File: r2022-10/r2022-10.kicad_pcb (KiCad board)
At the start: 4 copper layers, 100 x 80 mm, 137 parts, among them J1 Conn_01x03_Male, J2 USB_A male UP, J3 USB_B_Micro (up), J4 USB_A (female down), J5 USB_A_Stacked, J6 USB_A_Stacked, J7 USB_A_Stacked, J8 Conn_01x06, Q1 HSM6115, Q2 S8550, Q3 AO3401A, Q4 S8550, U1 2k i2c eeprom, U10 APL3511C, U11 NUP4202, U12 NUP4202, U13 NUP4202, U14 NUP4202, U15 NUP4202, U16 NUP4202, U17 NUP4202, U18 SiC437AED, U19 AMS1117-33, U2 NUP4202, U3 USB2517, U4 APL3511C, U5 APL3511C, U6 APL3511C, U7 APL3511C, U8 APL3511C, U9 APL3511C, Y1 24MHz

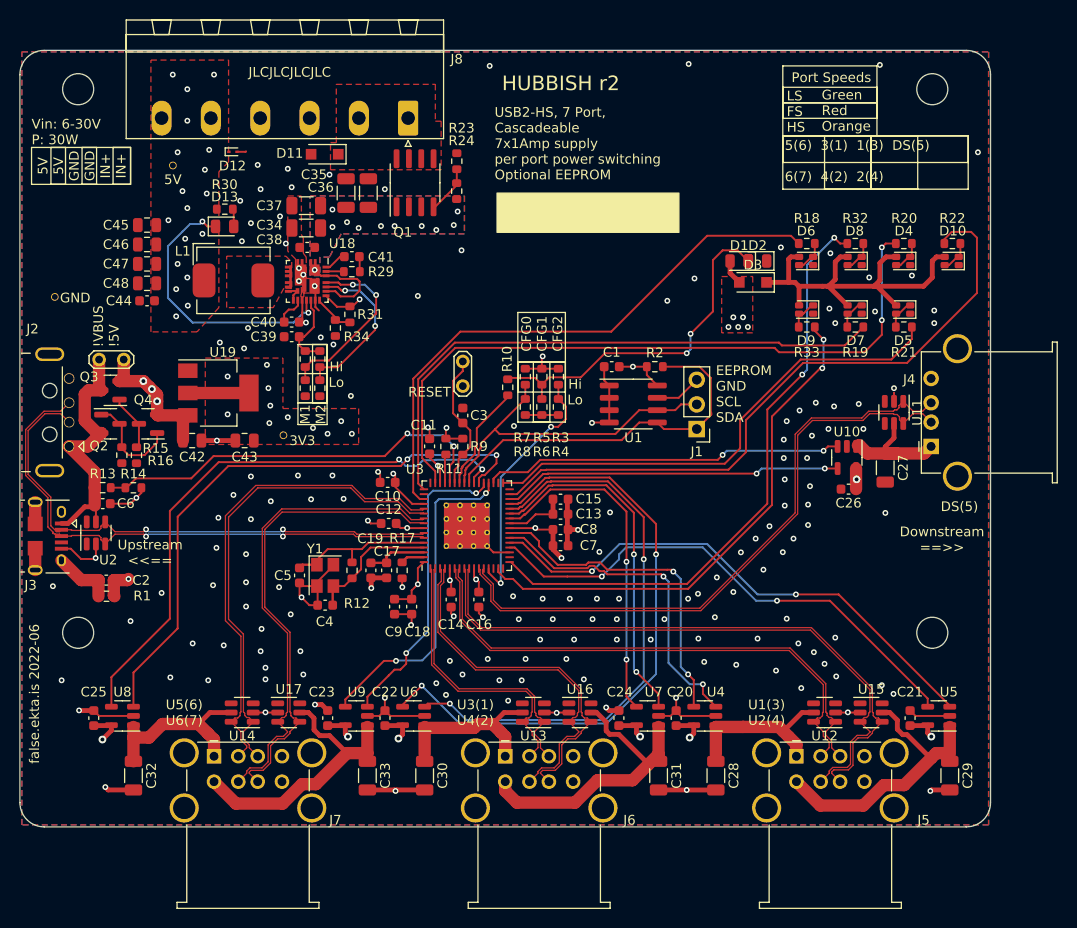
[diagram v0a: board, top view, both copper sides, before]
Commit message: r3: save all laast edits too
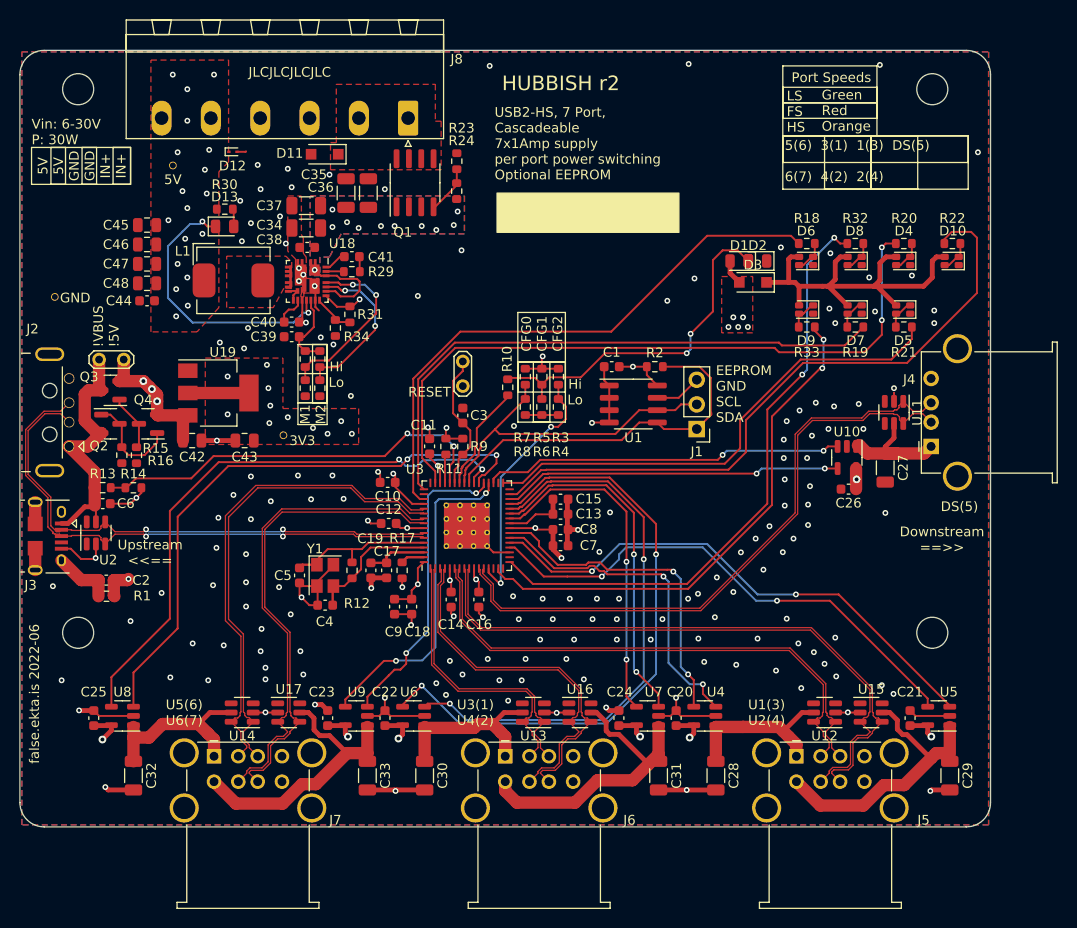
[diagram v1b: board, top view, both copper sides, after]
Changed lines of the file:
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@@
       (disableapertmacros false)
       (usegerberextensions false)
-      (usegerberattributes true)
+      (usegerberattributes false)
       (usegerberadvancedattributes true)
       (creategerberjobfile true)
@@
     (fp_line (start -1.6 -0.8) (end 1.6 -0.8) (layer "F.Fab") (width 0.1))
     (fp_line (start -1.6 0.8) (end -1.6 -0.8) (layer "F.Fab") (width 0.1))
-    (pad "1" smd roundrect (at -1.475 0 90) (size 1.15 1.8) (layers "F.Cu" "F.Paste" "F.Mask") (roundrect_rratio 0.217391)
+    (pad "1" smd roundrect (at -1.475 0 90) (size 1.15 1.8) (layers "F.Cu" "F.Paste" "F.Mask") (roundrect_rratio 0.2173913043)
       (net 14 "+VDC") (pintype "passive"))
-    (pad "2" smd roundrect (at 1.475 0 90) (size 1.15 1.8) (layers "F.Cu" "F.Paste" "F.Mask") (roundrect_rratio 0.217391)
+    (pad "2" smd roundrect (at 1.475 0 90) (size 1.15 1.8) (layers "F.Cu" "F.Paste" "F.Mask") (roundrect_rratio 0.2173913043)
       (net 1 "GND") (pintype "passive"))
     (model "${KICAD6_3DMODEL_DIR}/Capacitor_SMD.3dshapes/C_1206_3216Metric.wrl"
@@
     (fp_line (start 1.6 0.8) (end -1.6 0.8) (layer "F.Fab") (width 0.1))
     (fp_line (start -1.6 -0.8) (end 1.6 -0.8) (layer "F.Fab") (width 0.1))
-    (pad "1" smd roundrect (at -1.475 0 270) (size 1.15 1.8) (layers "F.Cu" "F.Paste" "F.Mask") (roundrect_rratio 0.217391)
+    (pad "1" smd roundrect (at -1.475 0 270) (size 1.15 1.8) (layers "F.Cu" "F.Paste" "F.Mask") (roundrect_rratio 0.2173913043)
       (net 9 "/downstream-port-power/VBUS2") (pintype "passive"))
-    (pad "2" smd roundrect (at 1.475 0 270) (size 1.15 1.8) (layers "F.Cu" "F.Paste" "F.Mask") (roundrect_rratio 0.217391)
+    (pad "2" smd roundrect (at 1.475 0 270) (size 1.15 1.8) (layers "F.Cu" "F.Paste" "F.Mask") (roundrect_rratio 0.2173913043)
       (net 1 "GND") (pintype "passive"))
     (model "${KICAD6_3DMODEL_DIR}/Capacitor_SMD.3dshapes/C_1206_3216Metric.wrl"
@@
     (fp_line (start 1.6 -0.8) (end 1.6 0.8) (layer "F.Fab") (width 0.1))
     (fp_line (start -1.6 0.8) (end -1.6 -0.8) (layer "F.Fab") (width 0.1))
-    (pad "1" smd roundrect (at -1.475 0 270) (size 1.15 1.8) (layers "F.Cu" "F.Paste" "F.Mask") (roundrect_rratio 0.217391)
+    (pad "1" smd roundrect (at -1.475 0 270) (size 1.15 1.8) (layers "F.Cu" "F.Paste" "F.Mask") (roundrect_rratio 0.2173913043)
       (net 67 "/downstream-port-power/VBUS_DS") (pintype "passive"))
-    (pad "2" smd roundrect (at 1.475 0 270) (size 1.15 1.8) (layers "F.Cu" "F.Paste" "F.Mask") (roundrect_rratio 0.217391)
+    (pad "2" smd roundrect (at 1.475 0 270) (size 1.15 1.8) (layers "F.Cu" "F.Paste" "F.Mask") (roundrect_rratio 0.2173913043)
       (net 1 "GND") (pintype "passive"))
     (model "${KICAD6_3DMODEL_DIR}/Capacitor_SMD.3dshapes/C_1206_3216Metric.wrl"
@@
     (fp_line (start -1.6 -0.8) (end 1.6 -0.8) (layer "F.Fab") (width 0.1))
     (fp_line (start -1.6 0.8) (end -1.6 -0.8) (layer "F.Fab") (width 0.1))
-    (pad "1" smd roundrect (at -1.475 0 270) (size 1.15 1.8) (layers "F.Cu" "F.Paste" "F.Mask") (roundrect_rratio 0.217391)
+    (pad "1" smd roundrect (at -1.475 0 270) (size 1.15 1.8) (layers "F.Cu" "F.Paste" "F.Mask") (roundrect_rratio 0.2173913043)
       (net 11 "/downstream-port-power/VBUS4") (pintype "passive"))
-    (pad "2" smd roundrect (at 1.475 0 270) (size 1.15 1.8) (layers "F.Cu" "F.Paste" "F.Mask") (roundrect_rratio 0.217391)
+    (pad "2" smd roundrect (at 1.475 0 270) (size 1.15 1.8) (layers "F.Cu" "F.Paste" "F.Mask") (roundrect_rratio 0.2173913043)
       (net 1 "GND") (pintype "passive"))
     (model "${KICAD6_3DMODEL_DIR}/Capacitor_SMD.3dshapes/C_1206_3216Metric.wrl"
@@
     (fp_line (start -1.6 0.8) (end -1.6 -0.8) (layer "F.Fab") (width 0.1))
     (fp_line (start 1.6 0.8) (end -1.6 0.8) (layer "F.Fab") (width 0.1))
-    (pad "1" smd roundrect (at -1.475 0 180) (size 1.15 1.8) (layers "F.Cu" "F.Paste" "F.Mask") (roundrect_rratio 0.217391)
+    (pad "1" smd roundrect (at -1.475 0 180) (size 1.15 1.8) (layers "F.Cu" "F.Paste" "F.Mask") (roundrect_rratio 0.2173913043)
       (net 14 "+VDC") (pintype "passive"))
-    (pad "2" smd roundrect (at 1.475 0 180) (size 1.15 1.8) (layers "F.Cu" "F.Paste" "F.Mask") (roundrect_rratio 0.217391)
+    (pad "2" smd roundrect (at 1.475 0 180) (size 1.15 1.8) (layers "F.Cu" "F.Paste" "F.Mask") (roundrect_rratio 0.2173913043)
       (net 1 "GND") (pintype "passive"))
     (model "${KICAD6_3DMODEL_DIR}/Capacitor_SMD.3dshapes/C_1206_3216Metric.wrl"
@@
     (fp_line (start 1.6 0.8) (end -1.6 0.8) (layer "F.Fab") (width 0.1))
     (fp_line (start 1.6 -0.8) (end 1.6 0.8) (layer "F.Fab") (width 0.1))
-    (pad "1" smd roundrect (at -1.475 0 270) (size 1.15 1.8) (layers "F.Cu" "F.Paste" "F.Mask") (roundrect_rratio 0.217391)
+    (pad "1" smd roundrect (at -1.475 0 270) (size 1.15 1.8) (layers "F.Cu" "F.Paste" "F.Mask") (roundrect_rratio 0.2173913043)
       (net 12 "/downstream-port-power/VBUS5") (pintype "passive"))
-    (pad "2" smd roundrect (at 1.475 0 270) (size 1.15 1.8) (layers "F.Cu" "F.Paste" "F.Mask") (roundrect_rratio 0.217391)
+    (pad "2" smd roundrect (at 1.475 0 270) (size 1.15 1.8) (layers "F.Cu" "F.Paste" "F.Mask") (roundrect_rratio 0.2173913043)
       (net 1 "GND") (pintype "passive"))
     (model "${KICAD6_3DMODEL_DIR}/Capacitor_SMD.3dshapes/C_1206_3216Metric.wrl"
@@
     (fp_line (start 1.6 -0.8) (end 1.6 0.8) (layer "F.Fab") (width 0.1))
     (fp_line (start 1.6 0.8) (end -1.6 0.8) (layer "F.Fab") (width 0.1))
-    (pad "1" smd roundrect (at -1.475 0 180) (size 1.15 1.8) (layers "F.Cu" "F.Paste" "F.Mask") (roundrect_rratio 0.217391)
+    (pad "1" smd roundrect (at -1.475 0 180) (size 1.15 1.8) (layers "F.Cu" "F.Paste" "F.Mask") (roundrect_rratio 0.2173913043)
       (net 14 "+VDC") (pintype "passive"))
-    (pad "2" smd roundrect (at 1.475 0 180) (size 1.15 1.8) (layers "F.Cu" "F.Paste" "F.Mask") (roundrect_rratio 0.217391)
+    (pad "2" smd roundrect (at 1.475 0 180) (size 1.15 1.8) (layers "F.Cu" "F.Paste" "F.Mask") (roundrect_rratio 0.2173913043)
       (net 1 "GND") (pintype "passive"))
     (model "${KICAD6_3DMODEL_DIR}/Capacitor_SMD.3dshapes/C_1206_3216Metric.wrl"
@@
     (fp_line (start -1.6 -0.8) (end 1.6 -0.8) (layer "F.Fab") (width 0.1))
     (fp_line (start 1.6 -0.8) (end 1.6 0.8) (layer "F.Fab") (width 0.1))
-    (pad "1" smd roundrect (at -1.475 0 270) (size 1.15 1.8) (layers "F.Cu" "F.Paste" "F.Mask") (roundrect_rratio 0.217391)
+    (pad "1" smd roundrect (at -1.475 0 270) (size 1.15 1.8) (layers "F.Cu" "F.Paste" "F.Mask") (roundrect_rratio 0.2173913043)
       (net 8 "/downstream-port-power/VBUS1") (pintype "passive"))
-    (pad "2" smd roundrect (at 1.475 0 270) (size 1.15 1.8) (layers "F.Cu" "F.Paste" "F.Mask") (roundrect_rratio 0.217391)
+    (pad "2" smd roundrect (at 1.475 0 270) (size 1.15 1.8) (layers "F.Cu" "F.Paste" "F.Mask") (roundrect_rratio 0.2173913043)
       (net 1 "GND") (pintype "passive"))
     (model "${KICAD6_3DMODEL_DIR}/Capacitor_SMD.3dshapes/C_1206_3216Metric.wrl"
@@
     (fp_line (start 1.6 0.8) (end -1.6 0.8) (layer "F.Fab") (width 0.1))
     (fp_line (start -1.6 -0.8) (end 1.6 -0.8) (layer "F.Fab") (width 0.1))
-    (pad "1" smd roundrect (at -1.475 0 90) (size 1.15 1.8) (layers "F.Cu" "F.Paste" "F.Mask") (roundrect_rratio 0.217391)
+    (pad "1" smd roundrect (at -1.475 0 90) (size 1.15 1.8) (layers "F.Cu" "F.Paste" "F.Mask") (roundrect_rratio 0.2173913043)
       (net 14 "+VDC") (pintype "passive"))
-    (pad "2" smd roundrect (at 1.475 0 90) (size 1.15 1.8) (layers "F.Cu" "F.Paste" "F.Mask") (roundrect_rratio 0.217391)
+    (pad "2" smd roundrect (at 1.475 0 90) (size 1.15 1.8) (layers "F.Cu" "F.Paste" "F.Mask") (roundrect_rratio 0.2173913043)
       (net 1 "GND") (pintype "passive"))
     (model "${KICAD6_3DMODEL_DIR}/Capacitor_SMD.3dshapes/C_1206_3216Metric.wrl"
@@
     (fp_line (start 1.6 0.8) (end -1.6 0.8) (layer "F.Fab") (width 0.1))
     (fp_line (start -1.6 -0.8) (end 1.6 -0.8) (layer "F.Fab") (width 0.1))
-    (pad "1" smd roundrect (at -1.475 0 270) (size 1.15 1.8) (layers "F.Cu" "F.Paste" "F.Mask") (roundrect_rratio 0.217391)
+    (pad "1" smd roundrect (at -1.475 0 270) (size 1.15 1.8) (layers "F.Cu" "F.Paste" "F.Mask") (roundrect_rratio 0.2173913043)
       (net 16 "/downstream-port-power/VBUS6") (pintype "passive"))
-    (pad "2" smd roundrect (at 1.475 0 270) (size 1.15 1.8) (layers "F.Cu" "F.Paste" "F.Mask") (roundrect_rratio 0.217391)
+    (pad "2" smd roundrect (at 1.475 0 270) (size 1.15 1.8) (layers "F.Cu" "F.Paste" "F.Mask") (roundrect_rratio 0.2173913043)
       (net 1 "GND") (pintype "passive"))
     (model "${KICAD6_3DMODEL_DIR}/Capacitor_SMD.3dshapes/C_1206_3216Metric.wrl"
@@
     (fp_line (start 1.6 -0.8) (end 1.6 0.8) (layer "F.Fab") (width 0.1))
     (fp_line (start -1.6 0.8) (end -1.6 -0.8) (layer "F.Fab") (width 0.1))
-    (pad "1" smd roundrect (at -1.475 0 270) (size 1.15 1.8) (layers "F.Cu" "F.Paste" "F.Mask") (roundrect_rratio 0.217391)
+    (pad "1" smd roundrect (at -1.475 0 270) (size 1.15 1.8) (layers "F.Cu" "F.Paste" "F.Mask") (roundrect_rratio 0.2173913043)
       (net 10 "/downstream-port-power/VBUS3") (pintype "passive"))
-    (pad "2" smd roundrect (at 1.475 0 270) (size 1.15 1.8) (layers "F.Cu" "F.Paste" "F.Mask") (roundrect_rratio 0.217391)
+    (pad "2" smd roundrect (at 1.475 0 270) (size 1.15 1.8) (layers "F.Cu" "F.Paste" "F.Mask") (roundrect_rratio 0.2173913043)
       (net 1 "GND") (pintype "passive"))
     (model "${KICAD6_3DMODEL_DIR}/Capacitor_SMD.3dshapes/C_1206_3216Metric.wrl"
@@
   (via (at 133.6 130.7) (size 0.6) (drill 0.3) (layers "F.Cu" "B.Cu") (free) (net 1))
   (via (at 136.652 126.492) (size 0.6) (drill 0.3) (layers "F.Cu" "B.Cu") (free) (net 1))
-  (via (at 146.4 128.6) (size 0.6) (drill 0.3) (layers "F.Cu" "B.Cu") (free) (net 1))
+  (via (at 146.2 128.6) (size 0.6) (drill 0.3) (layers "F.Cu" "B.Cu") (free) (net 1))
   (via (at 161.8 132) (size 0.6) (drill 0.3) (layers "F.Cu" "B.Cu") (free) (net 1))
   (via (at 163.3 109) (size 0.6) (drill 0.3) (layers "F.Cu" "B.Cu") (free) (net 1))
